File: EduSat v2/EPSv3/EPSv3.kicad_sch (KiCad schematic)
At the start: 1 part

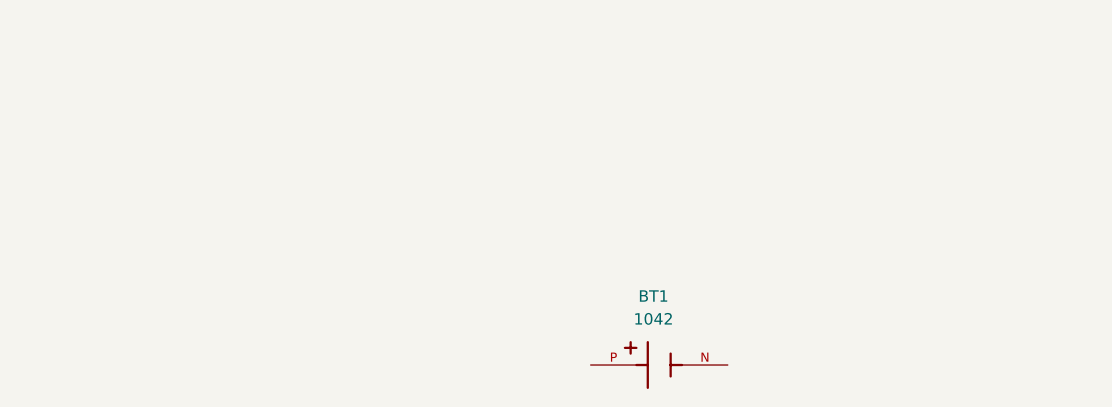
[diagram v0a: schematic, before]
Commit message: EPS updates
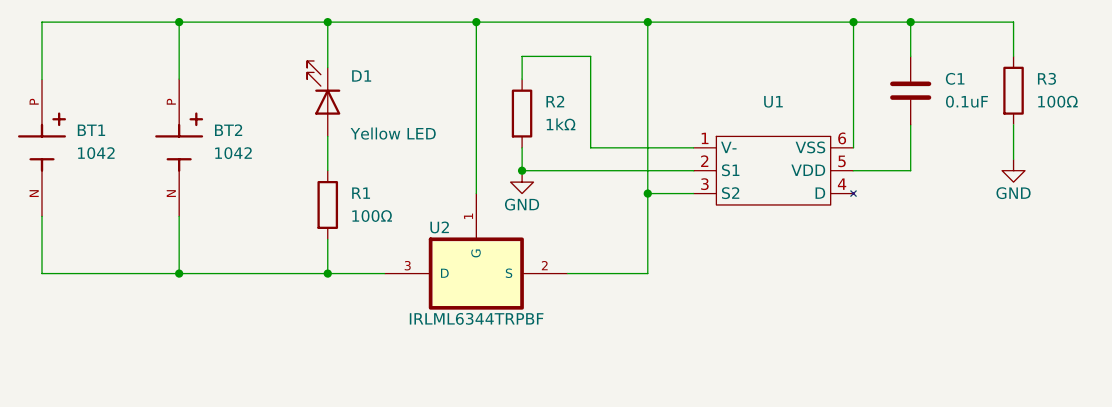
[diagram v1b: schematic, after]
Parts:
- removed BT1: 1042, BatteryHolderSingle:BAT_1042, symbol 1042:1042
- added BT1, BT2: 1042, Battery_Holder_1:BAT_1042, symbol Battery_Holder_1:1042
- added C1: 0.1uF, Capacitor_SMD:C_0805_2012Metric_Pad1.18x1.45mm_HandSolder, symbol Device:C
- added D1: Yellow LED, LED_SMD:LED_0805_2012Metric_Pad1.15x1.40mm_HandSolder, symbol Device:LED
- added R1, R3: 100Ω, Resistor_SMD:R_0805_2012Metric_Pad1.20x1.40mm_HandSolder, symbol Device:R
- added R2: 1kΩ, Resistor_SMD:R_0805_2012Metric_Pad1.20x1.40mm_HandSolder, symbol Device:R
- added U1: ~, DW06D:SOT-23-6_L2.9-W1.6-P0.95-LS2.8-BR, symbol DW06D:DW06D
- added U2: IRLML6344TRPBF, IRLML6344TRPBF:SOT95P240X112-3N, symbol IRLML6344TRPBF:IRLML6344TRPBF
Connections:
- new net: BT1.P, BT2.P, C1.1, D1.1 (K), R3.1, U1.3 (S2), U1.6 (VSS), U2.1 (G), U2.2 (S)
- new net: D1.2 (A), R1.1
- new net: BT1.N, BT2.N, R1.2, U2.3 (D)
- new net: R2.1, U1.1 (V-)
- new net: C1.2, U1.5 (VDD)
- new net GND: R2.2, R3.2, U1.2 (S1)
